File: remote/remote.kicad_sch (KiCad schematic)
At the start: 11 parts, among them J1 Conn_Coaxial, SW1 SW_SPST, U1 RFM69W, U2 PIC12LF1552

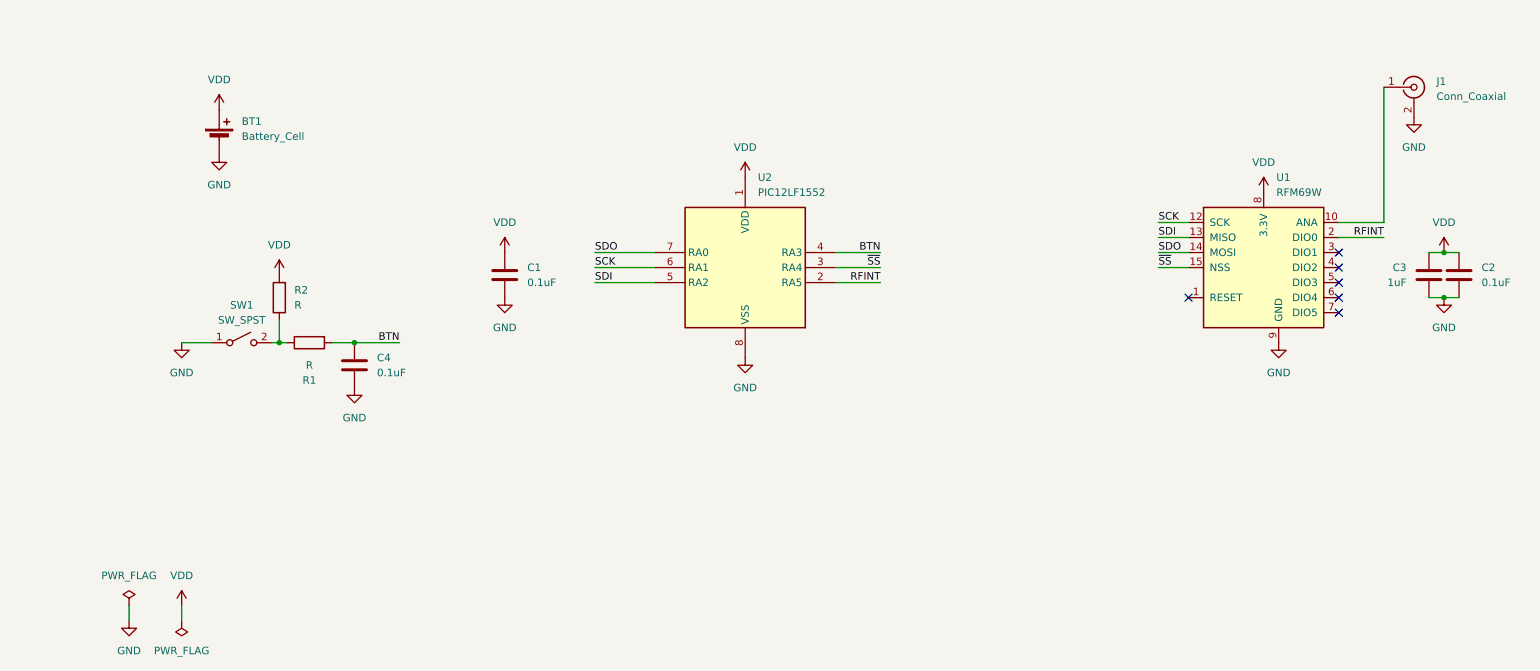
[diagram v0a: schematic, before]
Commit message: Base board Rev3
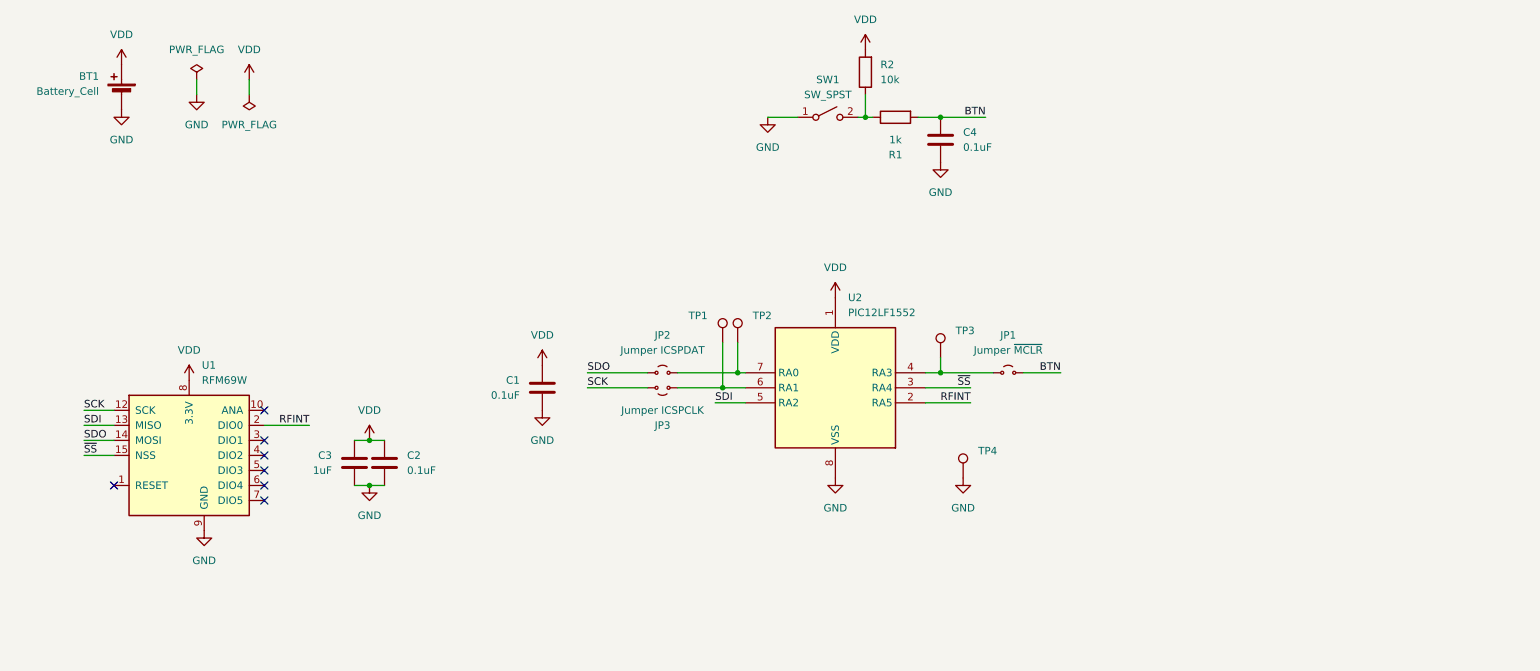
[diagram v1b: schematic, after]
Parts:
- removed J1: Conn_Coaxial, Connector_Coaxial:U.FL_Hirose_U.FL-R-SMT-1_Vertical, symbol Connector:Conn_Coaxial
- added JP1: Jumper ~{MCLR}, Jumper:SolderJumper-2_P1.3mm_Open_RoundedPad1.0x1.5mm, symbol Jumper:Jumper_2_Small_Open
- added JP2: Jumper ICSPDAT, Jumper:SolderJumper-2_P1.3mm_Open_RoundedPad1.0x1.5mm, symbol Jumper:Jumper_2_Small_Open
- added JP3: Jumper ICSPCLK, Jumper:SolderJumper-2_P1.3mm_Open_RoundedPad1.0x1.5mm, symbol Jumper:Jumper_2_Small_Open
- added TP1, TP2, TP3, TP4: TestPoint, TestPoint:TestPoint_Keystone_5000-5004_Miniature, symbol Connector:TestPoint
- C1, C2, C4: footprint Capacitor_SMD:C_0402_1005Metric_Pad0.74x0.62mm_HandSolder -> Capacitor_SMD:C_0603_1608Metric_Pad1.08x0.95mm_HandSolder
- R1: value R -> 1k; footprint Resistor_SMD:R_0402_1005Metric_Pad0.72x0.64mm_HandSolder -> Resistor_SMD:R_0603_1608Metric_Pad0.98x0.95mm_HandSolder
- R2: value R -> 10k; footprint Resistor_SMD:R_0402_1005Metric_Pad0.72x0.64mm_HandSolder -> Resistor_SMD:R_0603_1608Metric_Pad0.98x0.95mm_HandSolder
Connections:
- net BTN: now also JP1.2 (B); no longer U2.4 (RA3)
- net GND: now also TP4.1
- net SCK: now also JP3.1 (A); no longer U2.6 (RA1)
- net SDO: now also JP2.1 (A); no longer U2.7 (RA0)
- new net: JP1.1 (A), TP3.1, U2.4 (RA3)
- new net: JP2.2 (B), TP2.1, U2.7 (RA0)
- new net: JP3.2 (B), TP1.1, U2.6 (RA1)
- no-connect marks 6 -> 7
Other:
- moved on the sheet: BT1, C1, C2, C3, C4, R1, R2, SW1, U1, U2
